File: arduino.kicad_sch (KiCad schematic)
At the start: 11 parts, among them J2 Carte_Relais, J4 Conn_01x08_P2.54mm_pinheader_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, J6 Conn_01x02, J7 Con_01x03, U1 WX-DC12003

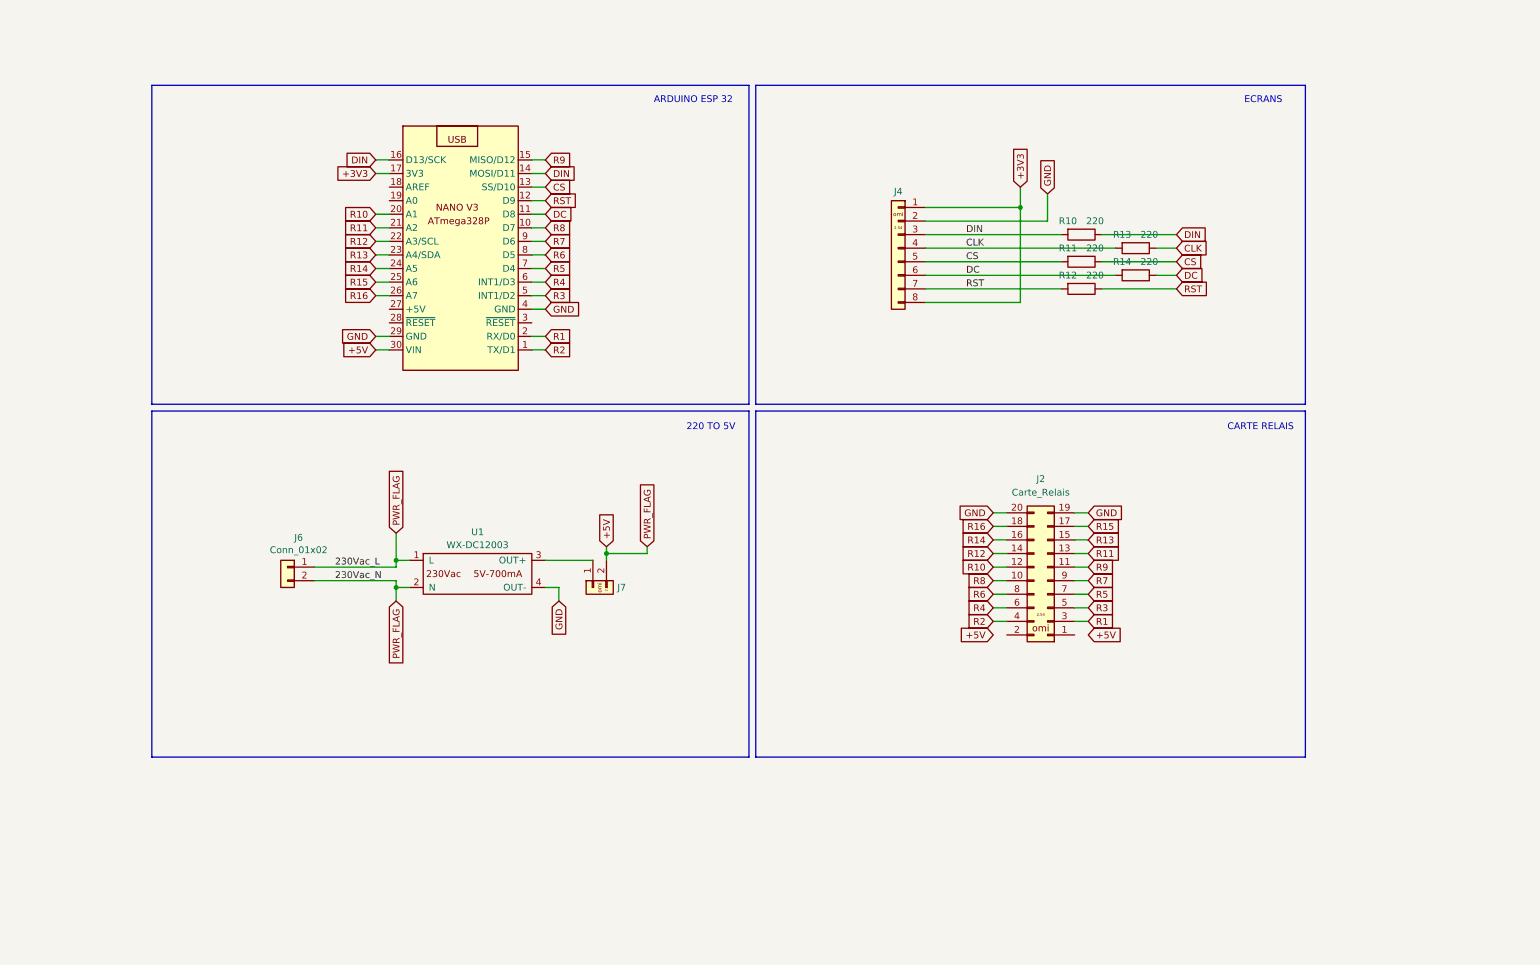
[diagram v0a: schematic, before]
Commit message: version 26/06/2025 08:31
Signed-off-by: TEST-BANC <TEST-BANC@DOMOMICRON.LOCAL>
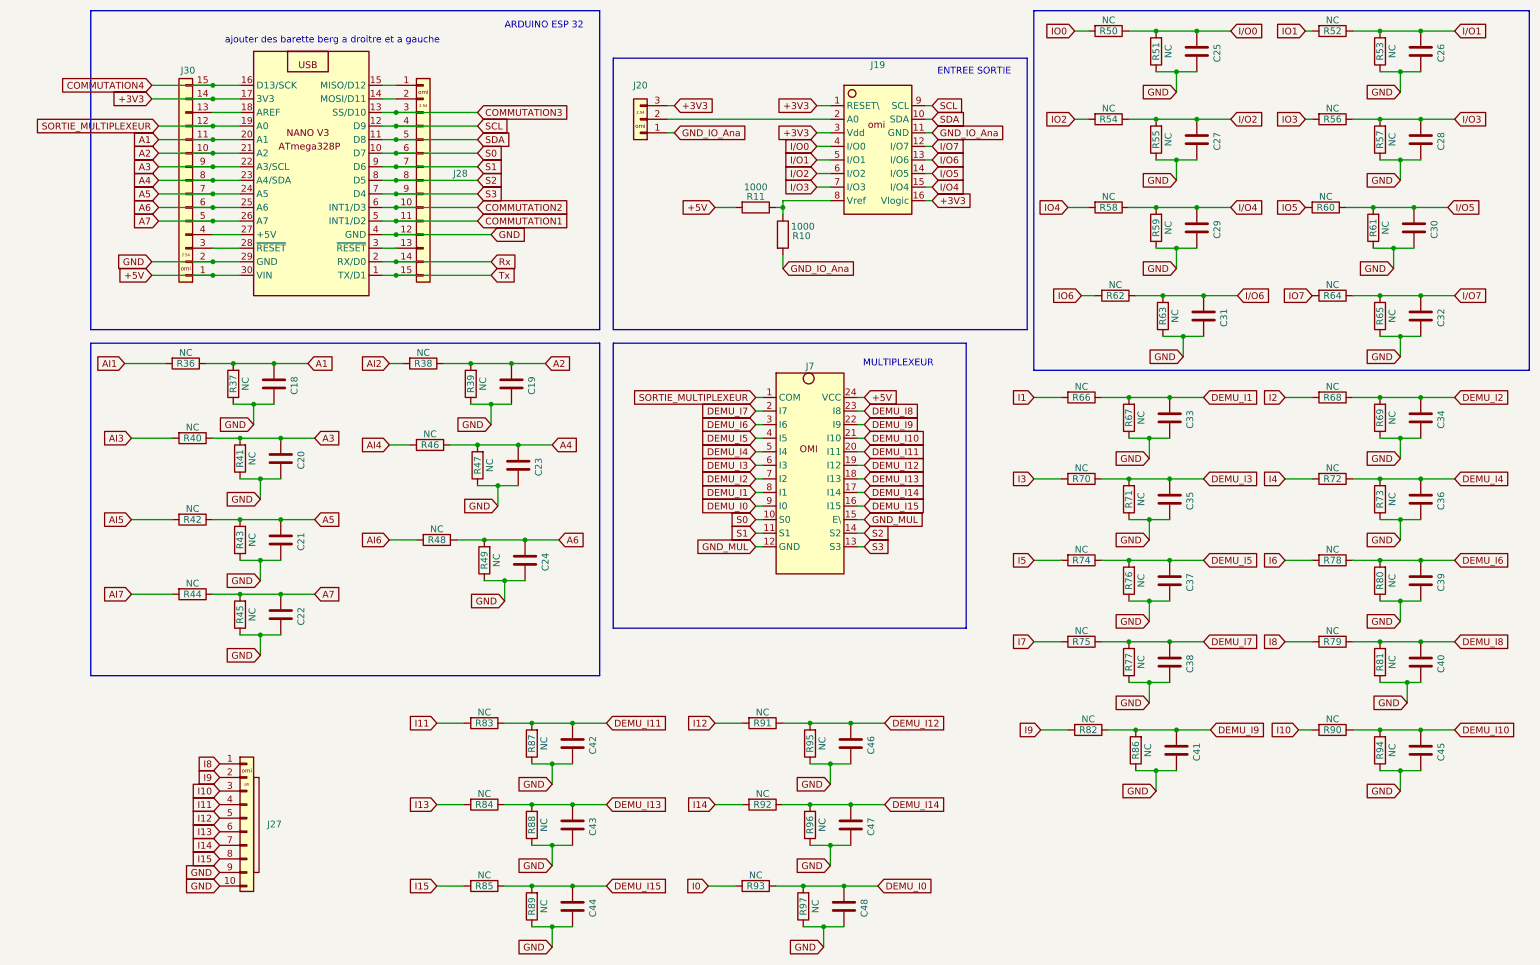
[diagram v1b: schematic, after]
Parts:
- removed J2: Carte_Relais, Omiconnecteur:PinHeader_2x10_P2.54mm_V_omi, symbol Omiconnecteur:Conn_02x10_Odd_Even_omi
- removed J4: Conn_01x08_P2.54mm_pinheader_vertical, Omiconnecteur:PinHeader_1x08_P2.54mm_V_omi, symbol Omiconnecteur:Conn_01x08_P2.54mm_pinheader_vertical
- removed J6: Conn_01x02, Connector_Phoenix_MC_HighVoltage:PhoenixContact_MCV_1,5_2-G-5.08_1x02_P5.08mm_Vertical, symbol Connector_Generic:Conn_01x02
- removed J7: Con_01x03, Omiconnecteur:PinHeader_1x02_P2.54mm_V_omi, symbol Omiconnecteur:Conn_01x02_P2.54mm_pinheader_vertical
- removed R12, R13, R14: 220, Resistor_SMD:R_0603_1608Metric_Pad0.98x0.95mm_HandSolder, symbol Device:R
- removed U1: WX-DC12003, Omievalboard:WX-DC12003, symbol Omievalboard:Omi_WX-DC12003
- added C18, C19, C20, C21, C22, C23, C24, C25, C26, C27, C28, C29, C30, C31, C32, C33, C34, C35, C36, C37, C38, C39, C40, C41, C42, C43, C44, C45, C46, C47, C48: C, symbol Device:C
- added J19: ~, symbol Omimultiplexeurs:AD5593R
- added J20: Con_01x03, Omiconnecteur:PinHeader_1x03_P2.54mm_V_omi, symbol Omiconnecteur:Conn_01x03_P2.54mm_pinheader_vertical
- added J27: Conn_PH_01x10, symbol Omiconnecteur:Conn_PH_01x10_P2.00mm_trad_vertical
- added J28, J30: Conn_01x32, Omiconnecteur:PinHeader_1x15_P2.54mm_V_omi, symbol Omiconnecteur:Conn_01x15_P2.54mm_pinheader_vertical
- added J7: CD74HC4067M96, symbol Omimultiplexeurs:CD74HC4067M96
- added R36, R37, R38, R39, R40, R41, R42, R43, R44, R45, R46, R47, R48, R49, R50, R51, R52, R53, R54, R55, R56, R57, R58, R59, R60, R61, R62, R63, R64, R65, R66, R67, R68, R69, R70, R71, R72, R73, R74, R75, R76, R77, R78, R79, R80, R81, R82, R83, R84, R85, R86, R87, R88, R89, R90, R91, R92, R93, R94, R95, R96, R97: NC, symbol Device:R
- R10, R11: value 220 -> 1000; footprint Resistor_SMD:R_0603_1608Metric_Pad0.98x0.95mm_HandSolder -> (none); Omicron 0603220E -> (none)
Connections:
- net +3V3: now also J19.1 (RESET\), J19.16 (Vlogic), J19.3 (Vdd), J20.3 (Pin_3), J30.14 (Pin_14)
- net +5V: now also R11.2, J30.1 (Pin_1), J7.24 (VCC)
- net GND: now also C18.2, C19.2, C20.2, C21.2, C22.2, C23.2, C24.2, C25.2, C26.2, C27.2, C28.2, C29.2, C30.2, C31.2, C32.2, C33.2, C34.2, C35.2, C36.2, C37.2, C38.2, C39.2, C40.2, C41.2, C42.2, C43.2, C44.2, C45.2, C46.2, C47.2, C48.2, J27.10 (Pin_10), J27.9 (Pin_9), J28.12 (Pin_12), J30.2 (Pin_2), R37.1, R39.1, R41.1, R43.1, R45.1, R47.1, R49.1, R51.1, R53.1, R55.1, R57.1, R59.1, R61.1, R63.1, R65.1, R67.1, R69.1, R71.1, R73.1, R76.1, R77.1, R80.1, R81.1, R86.1, R87.1, R88.1, R89.1, R94.1, R95.1, R96.1, R97.1
- net at A1.18 (AREF): now also J30.13 (Pin_13)
- net SORTIE_MULTIPLEXEUR: now reaches A1.19 (A0)
- net SORTIE_MULTIPLEXEUR: now also J30.12 (Pin_12), J7.1 (COM)
- net at A1.27 (+5V): now also J30.4 (Pin_4)
- net at A1.28 (~{RESET}): now also J30.3 (Pin_3)
- net at A1.3 (~{RESET}): now also J28.13 (Pin_13)
- removed net CS: A1.13 (SS/D10), R11.1, R11.2
- net DC renamed SDA
- net SDA: now also J19.10 (SDA), J28.5 (Pin_5)
- removed net DIN: A1.14 (MOSI/D11), A1.16 (D13/SCK), R10.1, R10.2
- net R1 renamed Rx
- net Rx: now also J28.14 (Pin_14)
- net R10 renamed A1
- net A1: now also C18.1, J30.11 (Pin_11), R36.1, R37.2
- net R11 renamed A2
- net A2: now also C19.1, J30.10 (Pin_10), R38.1, R39.2
- net R12 renamed A3
- net A3: now also C20.1, J30.9 (Pin_9), R40.1, R41.2
- net R13 renamed A4
- net A4: now also C23.1, J30.8 (Pin_8), R46.1, R47.2
- net R14 renamed A5
- net A5: now also C21.1, J30.7 (Pin_7), R42.1, R43.2
- net R15 renamed A6
- net A6: now also C24.1, J30.6 (Pin_6), R48.1, R49.2
- net R16 renamed A7
- net A7: now also C22.1, J30.5 (Pin_5), R44.1, R45.2
- net R2 renamed Tx
- net Tx: now also J28.15 (Pin_15)
- net R3 renamed COMMUTATION1
- net COMMUTATION1: now also J28.11 (Pin_11)
- net R4 renamed COMMUTATION2
- net COMMUTATION2: now also J28.10 (Pin_10)
- net R5 renamed S3
- net S3: now also J28.9 (Pin_9), J7.13 (S3)
- net R6 renamed S2
- net S2: now also J28.8 (Pin_8), J7.14 (S2)
- net R7 renamed S1
- net S1: now also J28.7 (Pin_7), J7.11 (S1)
- net R8 renamed S0
- net S0: now also J28.6 (Pin_6), J7.10 (S0)
- net R9: no longer names the net of A1.15 (MISO/D12)
- net R9: now also J28.1 (Pin_1)
- net RST renamed SCL
- net SCL: now also J19.9 (SCL), J28.4 (Pin_4)
- new net: J19.2 (A0), J20.2 (Pin_2)
- new net: J19.8 (Vref), R10.1, R11.1
- new net: A1.14 (MOSI/D11), J28.2 (Pin_2)
- new net AI1: R36.2
- new net AI2: R38.2
- new net AI3: R40.2
- new net AI4: R46.2
- new net AI5: R42.2
- new net AI6: R48.2
- new net AI7: R44.2
- new net COMMUTATION3: A1.13 (SS/D10), J28.3 (Pin_3)
- new net COMMUTATION4: A1.16 (D13/SCK), J30.15 (Pin_15)
- new net DEMU_I0: C48.1, J7.9 (I0), R93.1, R97.2
- new net DEMU_I1: C33.1, J7.8 (I1), R66.1, R67.2
- new net DEMU_I10: C45.1, J7.21 (I10), R90.1, R94.2
- new net DEMU_I11: C42.1, J7.20 (I11), R83.1, R87.2
- new net DEMU_I12: C46.1, J7.19 (I12), R91.1, R95.2
- new net DEMU_I13: C43.1, J7.18 (I13), R84.1, R88.2
- new net DEMU_I14: C47.1, J7.17 (I14), R92.1, R96.2
- new net DEMU_I15: C44.1, J7.16 (I15), R85.1, R89.2
- new net DEMU_I2: C34.1, J7.7 (I2), R68.1, R69.2
- new net DEMU_I3: C35.1, J7.6 (I3), R70.1, R71.2
- new net DEMU_I4: C36.1, J7.5 (I4), R72.1, R73.2
- new net DEMU_I5: C37.1, J7.4 (I5), R74.1, R76.2
- new net DEMU_I6: C39.1, J7.3 (I6), R78.1, R80.2
- new net DEMU_I7: C38.1, J7.2 (I7), R75.1, R77.2
- new net DEMU_I8: C40.1, J7.23 (I8), R79.1, R81.2
- new net DEMU_I9: C41.1, J7.22 (I9), R82.1, R86.2
- new net GND_IO_Ana: J19.11 (GND), J20.1 (Pin_1), R10.2
- new net GND_MUL: J7.12 (GND), J7.15 (E\)
- new net I0: R93.2
- new net I1: R66.2
- new net I10: J27.3 (Pin_3), R90.2
- new net I11: J27.4 (Pin_4), R83.2
- new net I12: J27.5 (Pin_5), R91.2
- new net I13: J27.6 (Pin_6), R84.2
- new net I14: J27.7 (Pin_7), R92.2
- new net I15: J27.8 (Pin_8), R85.2
- new net I2: R68.2
- new net I3: R70.2
- new net I4: R72.2
- new net I5: R74.2
- new net I6: R78.2
- new net I7: R75.2
- new net I8: J27.1 (Pin_1), R79.2
- new net I9: J27.2 (Pin_2), R82.2
- new net IO0: R50.2
- new net IO1: R52.2
- new net IO2: R54.2
- new net IO3: R56.2
- new net IO4: R58.2
- new net IO5: R60.2
- new net IO6: R62.2
- new net IO7: R64.2
- new net I/O0: C25.1, J19.4 (I/O0), R50.1, R51.2
- new net I/O1: C26.1, J19.5 (I/O1), R52.1, R53.2
- new net I/O2: C27.1, J19.6 (I/O2), R54.1, R55.2
- new net I/O3: C28.1, J19.7 (I/O3), R56.1, R57.2
- new net I/O4: C29.1, J19.15 (I/O4), R58.1, R59.2
- new net I/O5: C30.1, J19.14 (I/O5), R60.1, R61.2
- new net I/O6: C31.1, J19.13 (I/O6), R62.1, R63.2
- new net I/O7: C32.1, J19.12 (I/O7), R64.1, R65.2
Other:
- note added: "ENTREE SORTIE"
- note added: "MULTIPLEXEUR"
- note added: "ajouter des barette berg a droitre et a gauche"
- note removed: "220 TO 5V"
- note removed: "CARTE RELAIS"
- note removed: "ECRANS"
